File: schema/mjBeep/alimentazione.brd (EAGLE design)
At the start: 81 x 80 mm, 20 parts, among them IC1 LM317, IC2 LM350, IC3 7805T, J1 Alimentazione, J2 BATTERIA, J3 OUT, J4 OUT, T1 BC547

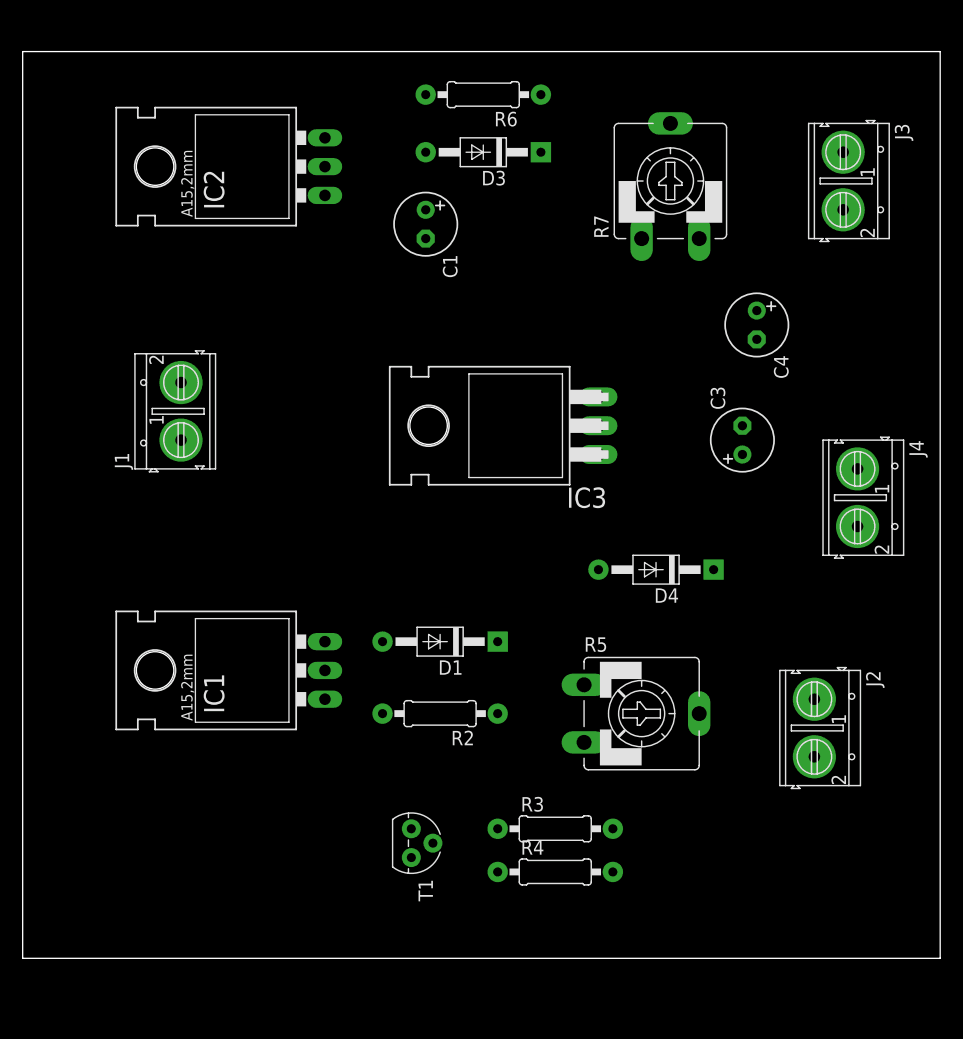
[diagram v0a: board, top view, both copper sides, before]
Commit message: mod
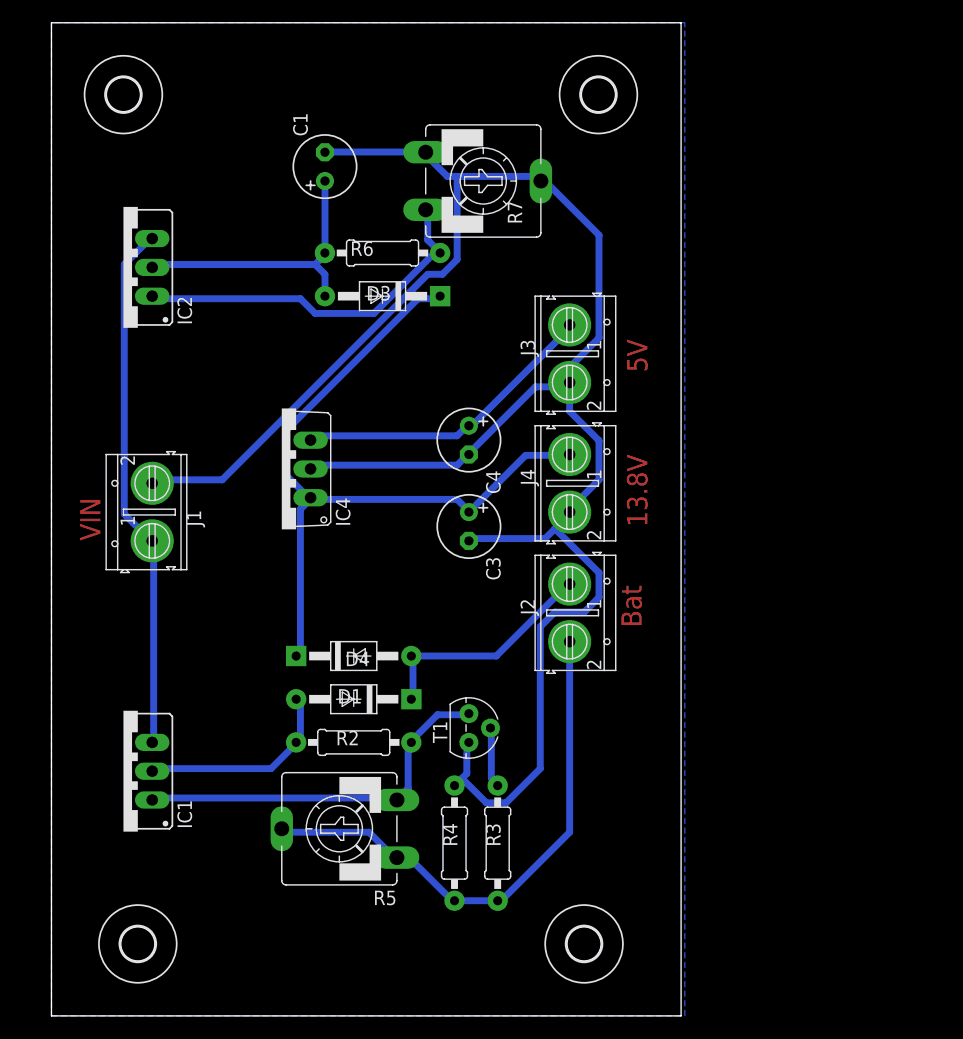
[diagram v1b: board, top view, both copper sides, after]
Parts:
- removed IC3: 7805T, linear:TO220H
- added IC4: 7805TV, linear:TO220V
- added U$1, U$2, U$3, U$4: (no value), holes:3,0
- IC1, IC2: device v-reg:317TL -> v-reg:317TS
- moved J3 28.5 mm to (43.2, 50.8)
- moved R5 28.5 mm to (22.9, 6.35), turned to 90 degrees
- moved D4 27.7 mm to (24.1, 21.6), turned to 0 degrees
- moved C4 27.4 mm to (34.3, 40.6)
- moved J4 25.4 mm to (43.2, 39.4)
- moved C3 25.3 mm to (34.3, 33.0), turned to 270 degrees
- moved J2 23.9 mm to (43.2, 27.9)
- moved R6 16.6 mm to (26.7, 57.1)
- moved IC1 16.6 mm to (3.81, 11.4)
- moved IC2 16.6 mm to (3.81, 55.9)
- moved R7 16.5 mm to (35.6, 63.5), turned to 270 degrees
- moved D3 15.5 mm to (26.7, 53.3)
- moved T1 11.4 mm to (34.3, 15.2)
- moved C1 10.2 mm to (21.6, 64.8), turned to 90 degrees
- moved J1 9.25 mm to (6.35, 31.8)
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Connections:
- net 13.8V: now also IC4.1; no longer IC3.1
- net 5V: now also IC4.3; no longer IC3.3
- net GND: now also IC4.2; no longer IC3.2
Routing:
- net GND: track 0.00 -> 173.4 mm
- net 13.8V: track 0.00 -> 65.7 mm
- net -BAT: track 0.00 -> 47.4 mm
- net N$13: track 0.00 -> 46.7 mm
- net N$27: track 0.00 -> 33.5 mm
- net N$5: track 0.00 -> 32.5 mm
- net 5V: track 0.00 -> 27.2 mm
- net N$3: track 0.00 -> 25.4 mm
- net +BAT: track 0.00 -> 20.6 mm
- net N$15: track 0.00 -> 18.2 mm
- net N$4: track 0.00 -> 5.32 mm
- added copper zone on layer 16, net N$1
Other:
- board size 81 x 80 mm -> 55.5 x 87.6 mm
- board text added: "13.8V"
- board text added: "5V"
- board text added: "Bat"
- board text added: "VIN"

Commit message: mod
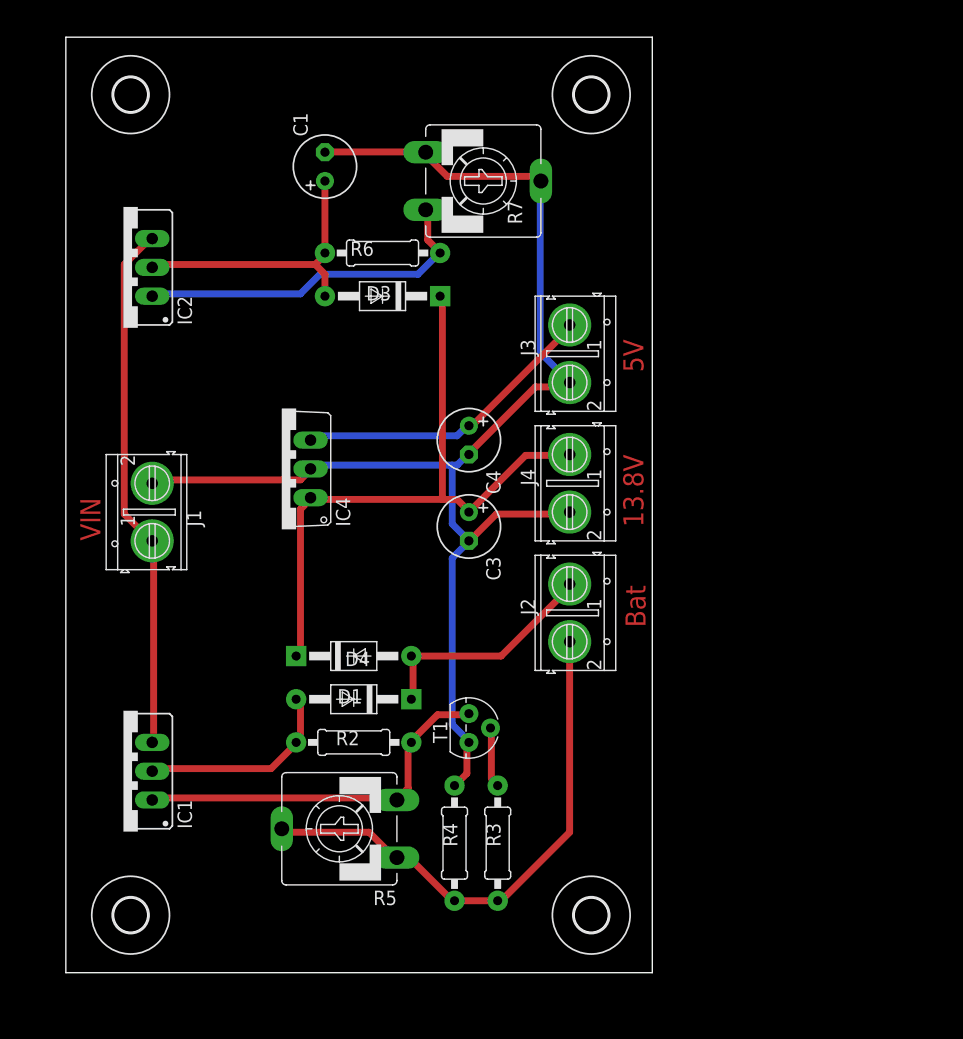
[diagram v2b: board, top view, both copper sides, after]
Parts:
- moved U$1 2.62 mm to (4.45, -1.27)
- moved U$2 2.62 mm to (45.1, -1.27)
- moved U$4 0.64 mm to (4.45, 71.1)
- moved U$3 0.63 mm to (45.1, 71.1)
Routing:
- net GND: track 173.4 -> 120.8 mm
- net 13.8V: track 65.7 -> 58.2 mm
- net N$5: track 32.5 -> 31.4 mm
- removed copper zone on layer 16, net N$1
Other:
- board size 55.5 x 87.6 mm -> 51.7 x 82.5 mm
